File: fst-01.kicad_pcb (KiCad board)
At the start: 2 copper layers, 21.2 x 12.6 mm, 17 parts, among them J1 USB_A, K1 CONN_3, U1 GD32F103TB, U2 MCP1700-3302E, U3 NUF2221W1, U4 X2SON, X1 12MHz

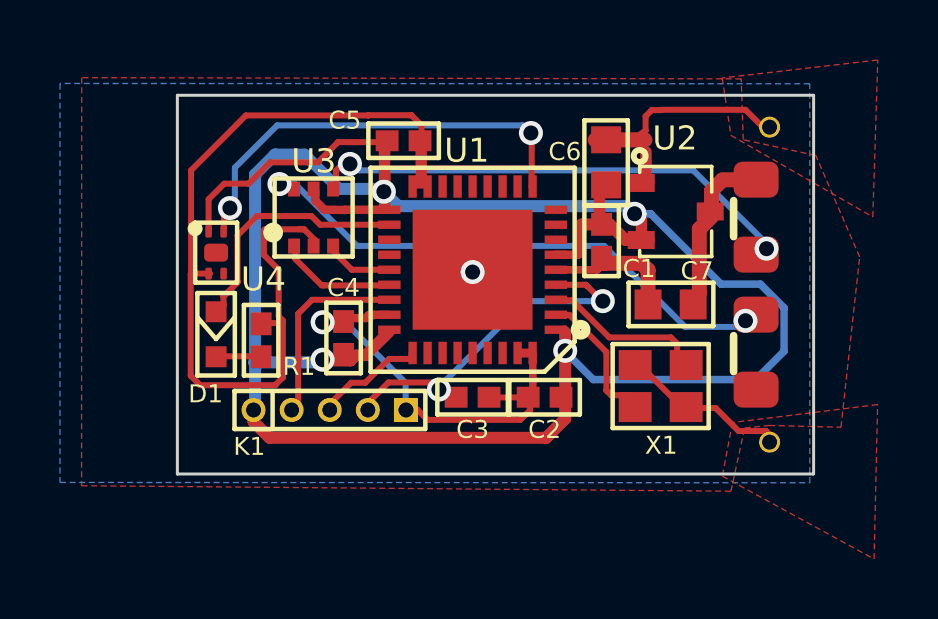
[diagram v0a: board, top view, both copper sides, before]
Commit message: Update PCBA.
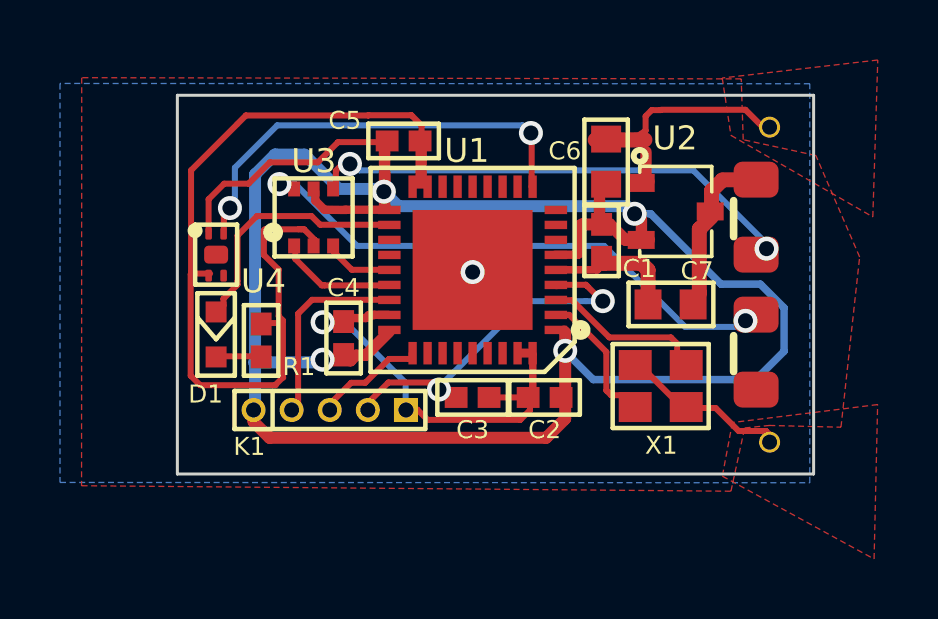
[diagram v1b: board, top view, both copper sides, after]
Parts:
- K1: value CONN_3 -> CONN_5
- U4: value X2SON -> DRV5032FA
- moved U4 0.07 mm to (109.8, 98.0)
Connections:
- U4 pad 3: (no net) -> Net-(U4-Pad3)
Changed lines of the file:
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@@
     (zones 0)
     (modules 17)
-    (nets 33)
+    (nets 34)
   )
   (page A4)
@@
   (net 31 "Net-(U1-Pad14)")
   (net 32 /PA3)
+  (net 33 "Net-(U4-Pad3)")
   (net_class Default "This is the default net class."
     (clearance 0.20066)
@@
     (add_net "Net-(U1-Pad8)")
     (add_net "Net-(U1-Pad9)")
+    (add_net "Net-(U4-Pad3)")
   )
   (net_class GND ""
@@
     (uvia_drill 0.14986)
   )
+  (module FST:X2SON (layer Front)
+    (at 109.75 97.9965)
+    (attr smd)
+    (fp_text reference U4 (at 1.5782 0.8887) (layer F.SilkS)
+      (effects (font (size 0.8 0.8) (thickness 0.15)))
+    )
+    (fp_text value DRV5032FA (at 0 -4.6) (layer F.Fab)
+      (effects (font (size 1 1) (thickness 0.15)))
+    )
+    (fp_line (start -0.55 -0.25) (end -0.1 -0.7) (layer Dwgs.User) (width 0.15))
+    (fp_circle (center -0.7 -0.8) (end -0.7 -0.7) (layer F.SilkS) (width 0.3))
+    (fp_line (start -0.7 -1) (end 0.7 -1) (layer F.SilkS) (width 0.15))
+    (fp_line (start 0.7 -1) (end 0.7 1) (layer F.SilkS) (width 0.15))
+    (fp_line (start 0.7 1) (end -0.7 1) (layer F.SilkS) (width 0.15))
+    (fp_line (start -0.7 1) (end -0.7 -1) (layer F.SilkS) (width 0.15))
+    (fp_line (start -0.55 -0.7) (end 0.55 -0.7) (layer Dwgs.User) (width 0.15))
+    (fp_line (start -0.55 0.7) (end 0.55 0.7) (layer Dwgs.User) (width 0.15))
+    (fp_line (start -0.55 -0.7) (end -0.55 0.7) (layer Dwgs.User) (width 0.15))
+    (fp_line (start 0.55 -0.7) (end 0.55 0.7) (layer Dwgs.User) (width 0.15))
+    (pad 5 smd roundrect (at 0 0) (size 0.8 0.6) (layers Front F.Paste F.Mask) (roundrect_rratio 0.25)
+      (solder_mask_margin 0.05) (solder_paste_margin -0.05) (clearance 0.05))
+    (pad 1 smd roundrect (at -0.25 -0.7) (size 0.22 0.4) (layers Front F.Paste F.Mask) (roundrect_rratio 0.25)
+      (net 13 +3V3) (solder_mask_margin 0.05) (clearance 0.05))
+    (pad 4 smd roundrect (at 0.25 -0.7) (size 0.22 0.4) (layers Front F.Paste F.Mask) (roundrect_rratio 0.25)
+      (net 32 /PA3) (solder_mask_margin 0.05) (clearance 0.05))
+    (pad 2 smd roundrect (at -0.25 0.7) (size 0.22 0.4) (layers Front F.Paste F.Mask) (roundrect_rratio 0.25)
+      (net 12 GND) (solder_mask_margin 0.05) (clearance 0.05))
+    (pad 3 smd roundrect (at 0.25 0.7) (size 0.22 0.4) (layers Front F.Paste F.Mask) (roundrect_rratio 0.25)
+      (net 33 "Net-(U4-Pad3)") (solder_mask_margin 0.05) (clearance 0.05))
+  )
   (module FST:SOT-23 (layer Front)
-    (at 125.0696 96.5581)
+    (at 125.07 96.5565)
     (descr "SOT-23, Standard")
     (tags SOT-23)
@@
   )
   (module FST:SOT363 (layer Front)
-    (at 113 96.76)
+    (at 113 96.7565)
     (descr "SMALL OUTLINE TRANSISTOR")
     (tags "SMALL OUTLINE TRANSISTOR")
@@
   )
   (module FST:FA-20H (layer Front)
-    (at 124.56922 102.37724)
+    (at 124.57 102.3765)
     (attr smd)
     (fp_text reference X1 (at 0.01778 1.97866) (layer F.SilkS)
@@
   )
   (module FST:LED0603 (layer Front)
-    (at 109.75 100.65 270)
+    (at 109.75 100.6565 270)
     (descr "LED 0603 smd package")
     (tags "LED led 0603 SMD smd SMT smt smdled SMDLED smtled SMTLED")
@@
       (effects (font (size 0.6 0.6) (thickness 0.15)))
     )
-    (fp_text value CONN_3 (at 0 -2.159) (layer F.SilkS) hide
+    (fp_text value CONN_5 (at 0 -2.159) (layer F.SilkS) hide
       (effects (font (size 1.016 1.016) (thickness 0.1524)))
     )
@@
   )
   (module FST:QFN36 (layer Front)
-    (at 118.3 98.5 180)
+    (at 118.3 98.5065 180)
     (descr "Support QFN 36 pins")
     (tags QFN36)
@@
       (net 12 GND) (solder_mask_margin 0.05) (solder_paste_margin -0.4699))
   )
-  (module FST:X2SON (layer Front)
-    (at 109.75 97.93)
-    (fp_text reference U4 (at 1.5782 0.8887) (layer F.SilkS)
-      (effects (font (size 0.8 0.8) (thickness 0.15)))
-    )
-    (fp_text value X2SON (at 0 -4.6) (layer F.Fab)
-      (effects (font (size 1 1) (thickness 0.15)))
-    )
-    (fp_line (start 0.55 -0.7) (end 0.55 0.7) (layer Dwgs.User) (width 0.15))
-    (fp_line (start -0.55 -0.7) (end -0.55 0.7) (layer Dwgs.User) (width 0.15))
-    (fp_line (start -0.55 0.7) (end 0.55 0.7) (layer Dwgs.User) (width 0.15))
-    (fp_line (start -0.55 -0.7) (end 0.55 -0.7) (layer Dwgs.User) (width 0.15))
-    (fp_line (start -0.7 1) (end -0.7 -1) (layer F.SilkS) (width 0.15))
-    (fp_line (start 0.7 1) (end -0.7 1) (layer F.SilkS) (width 0.15))
-    (fp_line (start 0.7 -1) (end 0.7 1) (layer F.SilkS) (width 0.15))
-    (fp_line (start -0.7 -1) (end 0.7 -1) (layer F.SilkS) (width 0.15))
-    (fp_circle (center -0.7 -0.8) (end -0.7 -0.7) (layer F.SilkS) (width 0.3))
-    (fp_line (start -0.55 -0.25) (end -0.1 -0.7) (layer Dwgs.User) (width 0.15))
-    (pad 3 smd roundrect (at 0.25 0.7) (size 0.22 0.4) (layers Front F.Paste F.Mask) (roundrect_rratio 0.25)
-      (solder_mask_margin 0.05) (clearance 0.05))
-    (pad 2 smd roundrect (at -0.25 0.7) (size 0.22 0.4) (layers Front F.Paste F.Mask) (roundrect_rratio 0.25)
-      (net 12 GND) (solder_mask_margin 0.05) (clearance 0.05))
-    (pad 4 smd roundrect (at 0.25 -0.7) (size 0.22 0.4) (layers Front F.Paste F.Mask) (roundrect_rratio 0.25)
-      (net 32 /PA3) (solder_mask_margin 0.05) (clearance 0.05))
-    (pad 1 smd roundrect (at -0.25 -0.7) (size 0.22 0.4) (layers Front F.Paste F.Mask) (roundrect_rratio 0.25)
-      (net 13 +3V3) (solder_mask_margin 0.05) (clearance 0.05))
-    (pad 5 smd roundrect (at 0 0) (size 0.8 0.6) (layers Front F.Paste F.Mask) (roundrect_rratio 0.25)
-      (solder_mask_margin 0.05) (solder_paste_margin -0.05) (clearance 0.05))
-  )
   (module FST:r_0402 (layer Front)
-    (at 111.25 100.85 270)
+    (at 111.25 100.8565 270)
     (descr "SMT resistor, 0402")
     (attr smd)
@@
   )
   (module FST:c_0603 (layer Front)
-    (at 124.9 99.6569)
+    (at 124.9 99.6565)
     (descr "SMT capacitor, 0603")
     (attr smd)
@@
   )
   (module FST:c_0402 (layer Front)
-    (at 122.6 97.536 270)
+    (at 122.6 97.5365 270)
     (descr "SMT capacitor, 0402")
     (attr smd)
@@
   )
   (module FST:c_0402 (layer Front)
-    (at 120.7 102.75 180)
+    (at 120.7 102.7565 180)
     (descr "SMT capacitor, 0402")
     (attr smd)
@@
   )
   (module FST:c_0402 (layer Front)
-    (at 116 94.2)
+    (at 116 94.2065)
     (descr "SMT capacitor, 0402")
     (attr smd)
@@
   )
   (module FST:c_0402 (layer Front)
-    (at 114 100.7745 90)
+    (at 114 100.7765 90)
     (descr "SMT capacitor, 0402")
     (attr smd)
@@
   )
   (module FST:c_0402 (layer Front)
-    (at 118.3 102.75 180)
+    (at 118.3 102.7565 180)
     (descr "SMT capacitor, 0402")
     (attr smd)
@@
   )
   (module FST:c_0603 (layer Front)
-    (at 122.75 94.92 270)
+    (at 122.75 94.8965 270)
     (descr "SMT capacitor, 0603")
     (attr smd)
@@
   (segment (start 112.9284 96.7105) (end 113.217831 96.999931) (width 0.20066) (layer Front) (net 5))
   (segment (start 110.4646 97.3582) (end 111.1123 96.7105) (width 0.20066) (layer Front) (net 5))
-  (segment (start 110.4646 98.9203) (end 110.4646 98.8822) (width 0.20066) (layer Front) (net 5))
-  (segment (start 109.9947 99.3902) (end 110.4646 98.9203) (width 0.20066) (layer Front) (net 5))
+  (segment (start 110.4646 98.9965) (end 110.4646 98.8822) (width 0.20066) (layer Front) (net 5))
+  (segment (start 109.9947 99.4664) (end 110.4646 98.9965) (width 0.20066) (layer Front) (net 5))
   (segment (start 109.8169 99.8728) (end 109.9947 99.695) (width 0.20066) (layer Front) (net 5))
-  (segment (start 109.9947 99.695) (end 109.9947 99.3902) (width 0.20066) (layer Front) (net 5))
+  (segment (start 109.9947 99.695) (end 109.9947 99.4664) (width 0.20066) (layer Front) (net 5))
   (segment (start 121.040808 99.001451) (end 121.090337 99.05098) (width 0.20066) (layer Front) (net 6) (status 30))
   (segment (start 121.040808 99.001451) (end 122.079891 99.001451) (width 0.20066) (layer Front) (net 6))
@@
   (segment (start 111.0488 95.32366) (end 111.71428 94.65818) (width 0.4) (layer Back) (net 13))
   (segment (start 111.05388 103.1875) (end 111.0488 103.18242) (width 0.4) (layer Back) (net 13))
-  (segment (start 111.0488 103.18242) (end 111.0488 95.32366) (width 0.4) (layer Back) (net 13))
+  (segment (start 111.0488 103.18242) (end 111.0488 95.31966) (width 0.4) (layer Back) (net 13))
   (segment (start 109.4994 96.1517) (end 109.4994 97.2185) (width 0.20066) (layer Front) (net 13))
   (segment (start 110.0201 95.631) (end 109.4994 96.1517) (width 0.20066) (layer Front) (net 13))
